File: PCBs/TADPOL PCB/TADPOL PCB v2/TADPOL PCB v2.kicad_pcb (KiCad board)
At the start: 2 copper layers, 56.5 x 65 mm, 17 parts

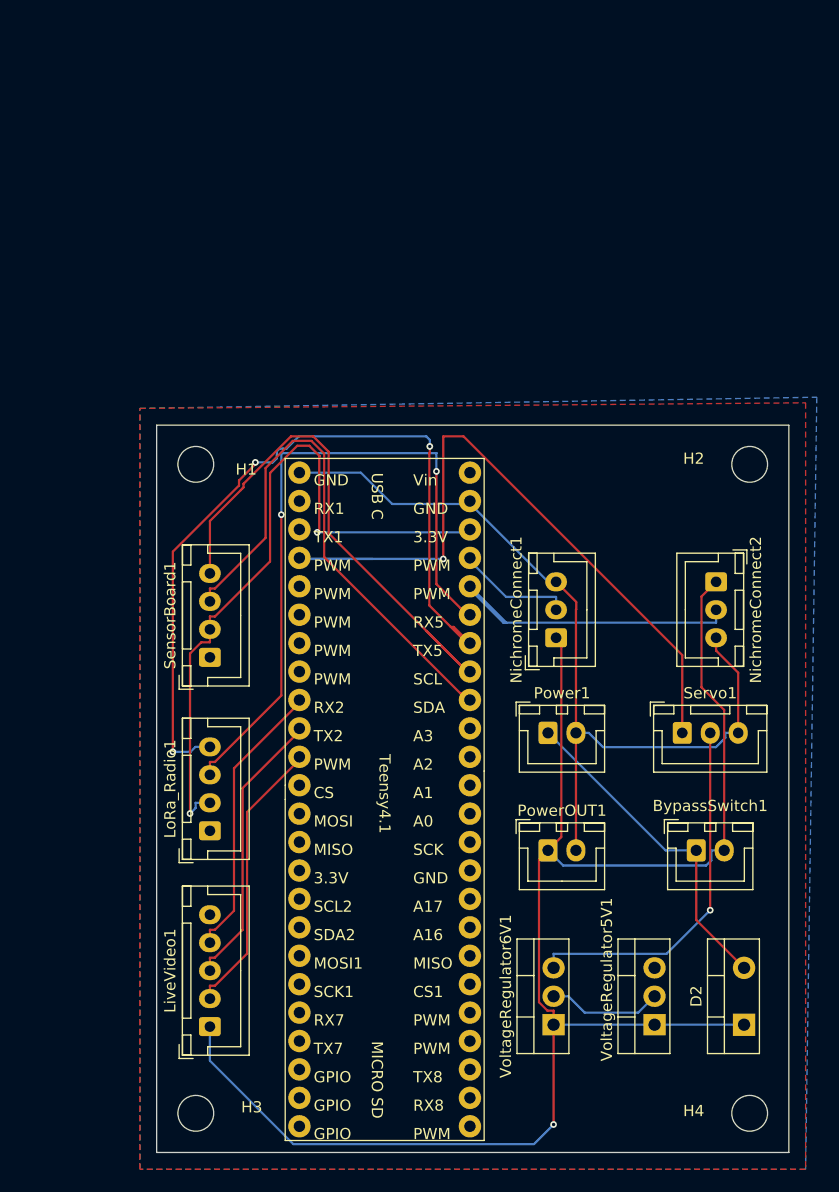
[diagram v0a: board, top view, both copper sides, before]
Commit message: Updated PCB
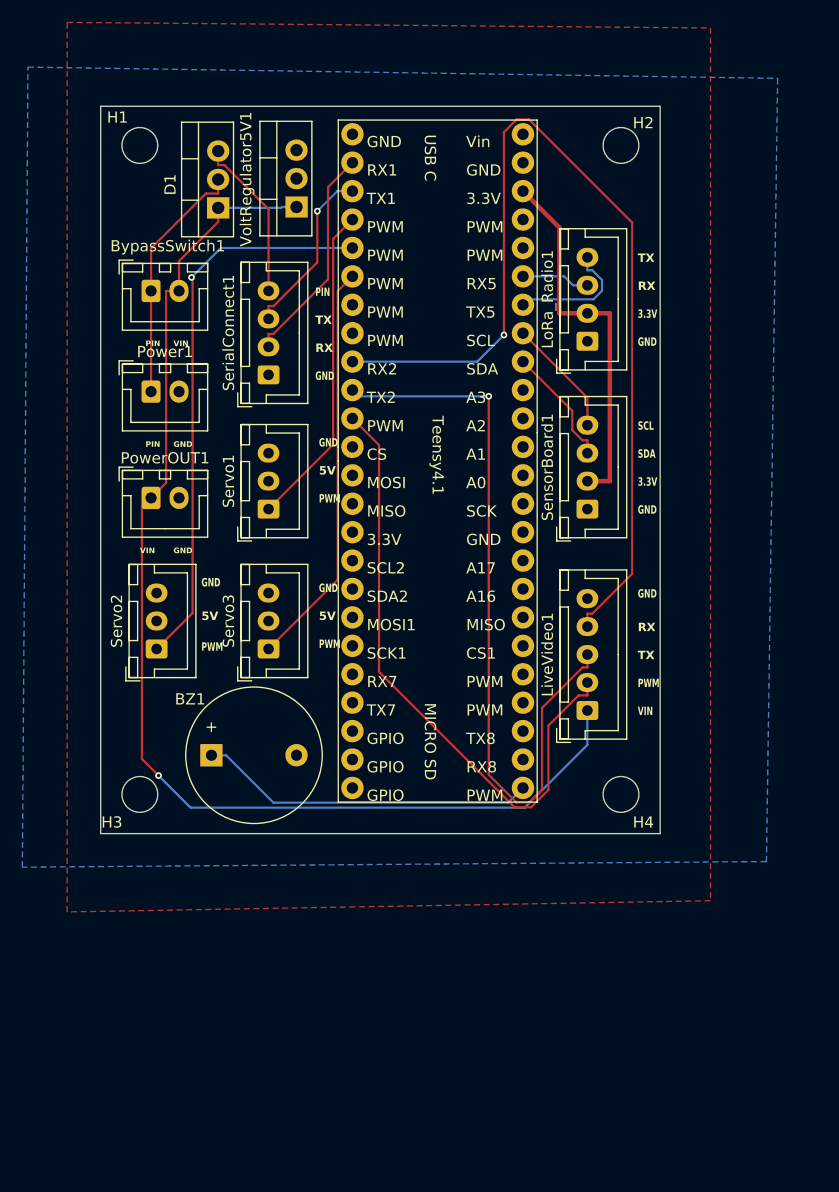
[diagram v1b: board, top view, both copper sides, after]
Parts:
- removed D2: D, Package_TO_SOT_THT:TO-220-2_Vertical
- removed NichromeConnect1, NichromeConnect2: Conn_01x03_Socket, Connector_JST:JST_XH_B3B-XH-A_1x03_P2.50mm_Vertical
- removed VoltageRegulator5V1: L7805, Package_TO_SOT_THT:TO-220-3_Vertical
- removed VoltageRegulator6V1: L7806, Package_TO_SOT_THT:TO-220-3_Vertical
- added BZ1: Buzzer, Buzzer_Beeper:Buzzer_12x9.5RM7.6, F.Cu at (125.9, 108.0)
- added D1: Q_SCR_KAG, Package_TO_SOT_THT:TO-220-3_Vertical, F.Cu at (126.5, 59.1)
- added G***: LOGO, LOGO, B.Cu at (146.5, 93.5)
- added SerialConnect1: Conn_01x04_Socket, Connector_JST:JST_XH_B4B-XH-A_1x04_P2.50mm_Vertical, F.Cu at (131.0, 74.0)
- added Servo2: Conn_01x03_Socket, Connector_JST:JST_XH_B3B-XH-A_1x03_P2.50mm_Vertical, F.Cu at (121.0, 98.5)
- added Servo3: Conn_01x03_Socket, Connector_JST:JST_XH_B3B-XH-A_1x03_P2.50mm_Vertical, F.Cu at (131.0, 98.5)
- added VoltRegulator5V1: L7805, Package_TO_SOT_THT:TO-220-3_Vertical, F.Cu at (133.5, 59.0)
- moved BypassSwitch1 69.8 mm to (120.5, 66.5)
- moved LoRa_Radio1 55.2 mm to (159.5, 71.0)
- moved PowerOUT1 47.4 mm to (120.5, 85.0)
- moved Power1 46.8 mm to (120.5, 75.5)
- moved LiveVideo1 44.0 mm to (159.5, 104.0)
- moved Servo1 42.0 mm to (131.0, 86.0), turned to 90 degrees
- moved SensorBoard1 36.2 mm to (159.5, 86.0)
- moved H2 30.7 mm to (162.5, 53.5)
- moved H4 30.7 mm to (162.5, 111.5)
- moved Teensy4.1 30.6 mm to (146.1, 81.7)
- moved H1 28.9 mm to (119.5, 53.5)
- moved H3 28.9 mm to (119.5, 111.5)
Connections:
- Servo1 pad 2: +6V -> +5V
- Teensy4.1 pad 1: unconnected-(Teensy4.1-RX1-Pad1) -> RX_SERIAL
- Teensy4.1 pad 2: unconnected-(Teensy4.1-TX1-Pad2) -> TX_SERIAL
- Teensy4.1 pad 24: unconnected-(Teensy4.1-PWM-Pad24) -> BUZZER
- Teensy4.1 pad 4: unconnected-(Teensy4.1-PWM-Pad4) -> PWM_SERVO2
- Teensy4.1 pad 43: PWM_NICHROME2 -> unconnected-(Teensy4.1-PWM-Pad43)
- Teensy4.1 pad 44: PWM_NICHROME1 -> unconnected-(Teensy4.1-PWM-Pad44)
- Teensy4.1 pad 5: unconnected-(Teensy4.1-PWM-Pad5) -> PWM_SERVO3
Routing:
- net GND: track 88.5 -> 0.00 mm
- net RX_VIDEO: track 25.3 -> 86.4 mm, vias 0 -> 1
- net TX_LORA: track 71.7 -> 11.4 mm, vias 3 -> 0
- net RX_LORA: track 62.6 -> 6.09 mm, vias 2 -> 0
- net PWM_SERVO2: track 0.00 -> 50.0 mm, vias 0 -> 1
- net TX_VIDEO: track 25.2 -> 66.5 mm, vias 0 -> 1
- net SCL: track 49.7 -> 10.6 mm
- net SDA: track 49.7 -> 10.8 mm
- net PWM_SERVO1: track 66.8 -> 29.0 mm, vias 1 -> 0
- net PWM_SERVO3: track 0.00 -> 36.4 mm
- net VIN: track 142.8 -> 106.8 mm
- net +6V: track 32.7 -> 0.00 mm, vias 1 -> 0
- net PWM_VIDEO: track 25.2 -> 55.9 mm
- net BUZZER: track 0.00 -> 30.1 mm
- net +3.3V: track 63.3 -> 33.8 mm, vias 2 -> 0
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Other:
- board size 56.5 x 65 mm -> 50 x 65 mm
- board text added: "3.3V"
- board text added: "5V"
- board text added: "GND"
- board text added: "PIN"
- board text added: "PWM"
- board text added: "RX"
- board text added: "SCL"
- board text added: "SDA"
- board text added: "TRT Payload PCB"
- board text added: "TX"
- board text added: "VIN"
